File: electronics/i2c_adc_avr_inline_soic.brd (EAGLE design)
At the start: 13.2 x 21.2 mm, 18 parts, among them IC1 TINY24/44/84-SSU, J1 AVRISP62LAYER, X1 PB2, X2 !SS, X3 PB0, X4 PA3

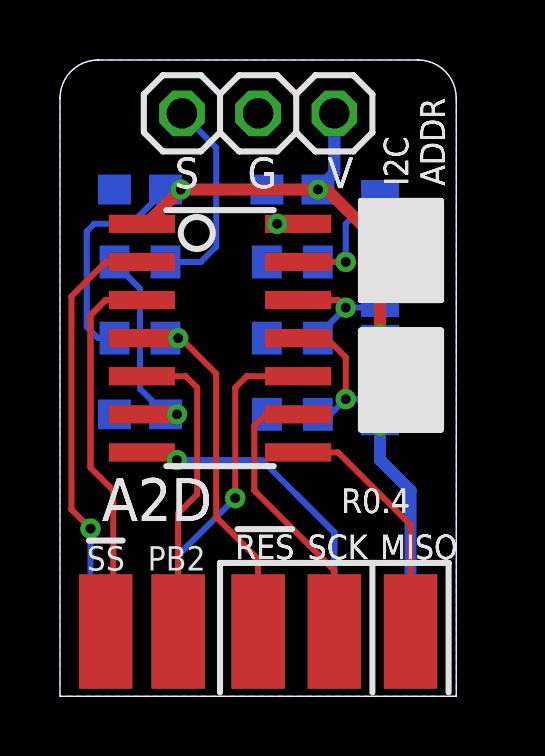
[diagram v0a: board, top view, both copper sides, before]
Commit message: Modified layouts, routing.
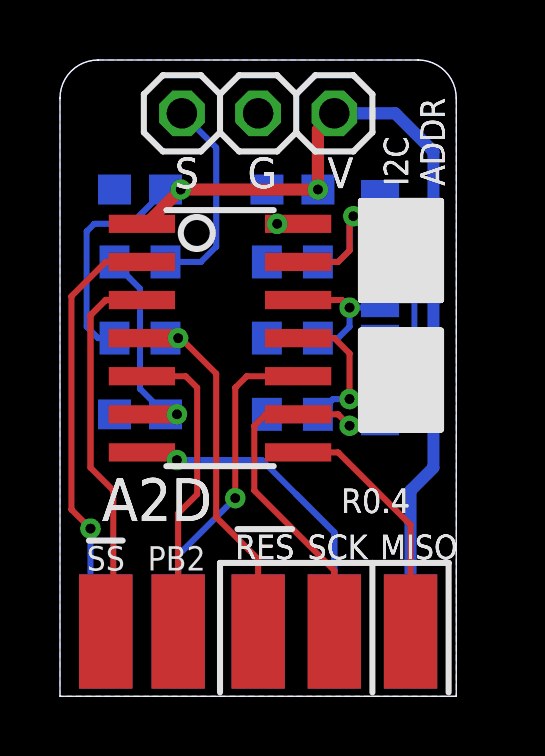
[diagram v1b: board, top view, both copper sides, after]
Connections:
- net TX/MISO: now also A0.3, A1.3, A2.3
- net VCC: no longer A0.3, A1.3, A2.3
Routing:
- net TX/MISO: track 8.30 -> 15.7 mm
- net VCC: track 34.0 -> 37.9 mm, vias 5 -> 2
- net SCL/SCK: track 9.58 -> 11.5 mm, vias 0 -> 1
- net A0: track 5.03 -> 6.37 mm
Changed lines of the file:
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@@
 <layer number="107" name="Crop" color="7" fill="1" visible="no" active="yes"/>
 <layer number="116" name="Patch_BOT" color="9" fill="4" visible="no" active="yes"/>
-<layer number="121" name="tsilk" color="14" fill="1" visible="yes" active="yes"/>
-<layer number="122" name="bsilk" color="6" fill="1" visible="yes" active="yes"/>
+<layer number="121" name="tsilk" color="14" fill="1" visible="no" active="yes"/>
+<layer number="122" name="bsilk" color="6" fill="1" visible="no" active="yes"/>
 <layer number="125" name="_tNames" color="7" fill="1" visible="no" active="yes"/>
 <layer number="144" name="Drill_legend" color="7" fill="1" visible="no" active="yes"/>
@@
 </signal>
 <signal name="VCC">
-<contactref element="A1" pad="3"/>
 <contactref element="C2" pad="1"/>
-<contactref element="A0" pad="3"/>
-<contactref element="A2" pad="3"/>
 <contactref element="C4" pad="1"/>
 <contactref element="R3" pad="2"/>
@@
 <wire x1="1.143" y1="15.748" x2="2.374" y2="15.748" width="0.2032" layer="16"/>
 <wire x1="2.374" y1="15.748" x2="3.517" y2="16.891" width="0.2032" layer="16"/>
-<wire x1="10.668" y1="7.874" x2="10.668" y2="9.017" width="0.4064" layer="16"/>
-<wire x1="9.144" y1="19.431" x2="9.144" y2="17.438" width="0.4064" layer="16"/>
-<wire x1="9.144" y1="17.438" x2="8.597" y2="16.891" width="0.4064" layer="16"/>
-<wire x1="10.668" y1="7.874" x2="11.684" y2="6.858" width="0.4064" layer="16"/>
-<via x="10.668" y="9.017" extent="1-16" drill="0.3302"/>
-<via x="10.668" y="12.065" extent="1-16" drill="0.3302"/>
-<via x="10.668" y="15.113" extent="1-16" drill="0.3302"/>
-<wire x1="10.668" y1="9.017" x2="10.668" y2="12.065" width="0.4064" layer="1"/>
-<wire x1="10.668" y1="12.065" x2="10.668" y2="15.113" width="0.4064" layer="1"/>
-<wire x1="10.668" y1="15.113" x2="8.89" y2="16.891" width="0.4064" layer="1"/>
-<wire x1="8.89" y1="16.891" x2="8.597" y2="16.891" width="0.4064" layer="1"/>
 <contactref element="J1" pad="VCC"/>
 <contactref element="J1" pad="VCC"/>
 <wire x1="11.684" y1="2.159" x2="11.684" y2="6.858" width="0.4064" layer="16"/>
+<wire x1="11.684" y1="6.858" x2="12.446" y2="7.62" width="0.4064" layer="16"/>
+<wire x1="12.446" y1="7.62" x2="12.446" y2="18.161" width="0.4064" layer="16"/>
+<wire x1="8.597" y1="16.891" x2="8.597" y2="18.884" width="0.4064" layer="1"/>
+<wire x1="8.597" y1="18.884" x2="9.144" y2="19.431" width="0.4064" layer="1"/>
+<wire x1="9.144" y1="19.431" x2="11.176" y2="19.431" width="0.4064" layer="16"/>
+<wire x1="11.176" y1="19.431" x2="12.446" y2="18.161" width="0.4064" layer="16"/>
 </signal>
 <signal name="GND">
@@
 <contactref element="R0" pad="2"/>
 <contactref element="IC1" pad="13"/>
-<wire x1="8.597" y1="14.478" x2="9.525" y2="14.478" width="0.2032" layer="16"/>
-<via x="9.525" y="14.478" extent="1-16" drill="0.3302"/>
-<wire x1="9.525" y1="14.478" x2="7.9375" y2="14.478" width="0.2032" layer="1"/>
-<wire x1="10.668" y1="16.002" x2="9.779" y2="16.002" width="0.2032" layer="16"/>
-<wire x1="9.779" y1="16.002" x2="9.525" y2="15.748" width="0.2032" layer="16"/>
-<wire x1="9.525" y1="15.748" x2="9.525" y2="14.478" width="0.2032" layer="16"/>
+<wire x1="8.597" y1="14.478" x2="9.271" y2="14.478" width="0.2032" layer="16"/>
+<wire x1="9.271" y1="14.478" x2="9.652" y2="14.859" width="0.2032" layer="16"/>
+<wire x1="9.652" y1="14.859" x2="9.652" y2="15.875" width="0.2032" layer="16"/>
+<wire x1="9.652" y1="15.875" x2="9.779" y2="16.002" width="0.2032" layer="16"/>
+<wire x1="9.779" y1="16.002" x2="10.668" y2="16.002" width="0.2032" layer="16"/>
+<wire x1="7.9375" y1="14.478" x2="9.271" y2="14.478" width="0.2032" layer="1"/>
+<wire x1="9.271" y1="14.478" x2="9.652" y2="14.859" width="0.2032" layer="1"/>
+<wire x1="9.652" y1="14.859" x2="9.652" y2="15.875" width="0.2032" layer="1"/>
+<wire x1="9.652" y1="15.875" x2="9.779" y2="16.002" width="0.2032" layer="1"/>
+<via x="9.779" y="16.002" extent="1-16" drill="0.3302"/>
 </signal>
 <signal name="A1">
@@
 <contactref element="R1" pad="2"/>
 <contactref element="IC1" pad="12"/>
-<wire x1="7.9375" y1="13.208" x2="9.271" y2="13.208" width="0.2032" layer="1"/>
-<wire x1="9.271" y1="13.208" x2="9.525" y2="12.954" width="0.2032" layer="1"/>
-<via x="9.525" y="12.954" extent="1-16" drill="0.3302"/>
-<wire x1="9.525" y1="12.954" x2="10.668" y2="12.954" width="0.2032" layer="16"/>
-<wire x1="8.597" y1="11.938" x2="8.509" y2="11.938" width="0.2032" layer="16"/>
-<wire x1="8.509" y1="11.938" x2="9.525" y2="12.954" width="0.2032" layer="16"/>
+<wire x1="8.597" y1="11.938" x2="9.271" y2="11.938" width="0.2032" layer="16"/>
+<wire x1="9.271" y1="11.938" x2="9.652" y2="12.319" width="0.2032" layer="16"/>
+<wire x1="9.652" y1="12.319" x2="9.652" y2="12.954" width="0.2032" layer="16"/>
+<wire x1="9.652" y1="12.954" x2="10.668" y2="12.954" width="0.2032" layer="16"/>
+<via x="9.652" y="12.954" extent="1-16" drill="0.3302"/>
+<wire x1="9.652" y1="12.954" x2="9.398" y2="13.208" width="0.2032" layer="1"/>
+<wire x1="9.398" y1="13.208" x2="7.9375" y2="13.208" width="0.2032" layer="1"/>
 </signal>
 <signal name="!RESET">
@@
 <wire x1="11.684" y1="2.159" x2="11.684" y2="5.715" width="0.2032" layer="1"/>
 <wire x1="11.684" y1="5.715" x2="9.271" y2="8.128" width="0.2032" layer="1"/>
+<contactref element="A1" pad="3"/>
+<contactref element="A0" pad="3"/>
+<contactref element="A2" pad="3"/>
+<wire x1="10.668" y1="9.017" x2="11.557" y2="9.017" width="0.2032" layer="16"/>
+<wire x1="11.557" y1="9.017" x2="11.811" y2="9.271" width="0.2032" layer="16"/>
+<wire x1="11.811" y1="9.271" x2="11.811" y2="12.192" width="0.2032" layer="16"/>
+<wire x1="11.811" y1="12.192" x2="11.811" y2="14.859" width="0.2032" layer="16"/>
+<wire x1="11.811" y1="14.859" x2="11.557" y2="15.113" width="0.2032" layer="16"/>
+<wire x1="11.684" y1="12.065" x2="11.811" y2="12.192" width="0.2032" layer="16"/>
+<wire x1="11.557" y1="15.113" x2="10.668" y2="15.113" width="0" layer="19" extent="16-16"/>
+<wire x1="10.668" y1="12.065" x2="11.684" y2="12.065" width="0" layer="19" extent="16-16"/>
+<wire x1="9.271" y1="8.128" x2="10.668" y2="9.017" width="0" layer="19" extent="1-16"/>
 </signal>
 <signal name="A2">
@@
 <contactref element="R2" pad="2"/>
 <contactref element="IC1" pad="11"/>
-<wire x1="10.668" y1="9.906" x2="9.525" y2="9.906" width="0.2032" layer="16"/>
-<wire x1="9.525" y1="9.906" x2="9.017" y2="9.398" width="0.2032" layer="16"/>
-<wire x1="9.017" y1="9.398" x2="8.597" y2="9.398" width="0.2032" layer="16"/>
-<wire x1="7.9375" y1="11.938" x2="8.89" y2="11.938" width="0.2032" layer="1"/>
-<wire x1="8.89" y1="11.938" x2="9.525" y2="11.303" width="0.2032" layer="1"/>
-<wire x1="9.525" y1="11.303" x2="9.525" y2="9.906" width="0.2032" layer="1"/>
-<via x="9.525" y="9.906" extent="1-16" drill="0.3302"/>
+<wire x1="10.668" y1="9.906" x2="9.652" y2="9.906" width="0.2032" layer="16"/>
+<wire x1="9.652" y1="9.906" x2="9.105" y2="9.906" width="0.2032" layer="16"/>
+<wire x1="9.105" y1="9.906" x2="8.597" y2="9.398" width="0.2032" layer="16"/>
+<wire x1="7.9375" y1="11.938" x2="9.144" y2="11.938" width="0.2032" layer="1"/>
+<wire x1="9.144" y1="11.938" x2="9.652" y2="11.43" width="0.2032" layer="1"/>
+<wire x1="9.652" y1="11.43" x2="9.652" y2="9.906" width="0.2032" layer="1"/>
+<via x="9.652" y="9.906" extent="1-16" drill="0.3302"/>
 </signal>
 <signal name="N$2">
@@
 <wire x1="9.144" y1="2.159" x2="9.144" y2="4.191" width="0.21701875" layer="1"/>
 <wire x1="6.477" y1="6.858" x2="9.144" y2="4.191" width="0.2032" layer="1"/>
+<wire x1="7.9375" y1="9.398" x2="9.271" y2="9.398" width="0.2032" layer="1"/>
+<wire x1="9.271" y1="9.398" x2="9.652" y2="9.017" width="0.2032" layer="1"/>
+<via x="9.652" y="9.017" extent="1-16" drill="0.3302"/>
 </signal>
 <signal name="!SS">
